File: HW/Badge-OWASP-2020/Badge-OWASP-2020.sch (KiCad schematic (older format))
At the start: 18 parts

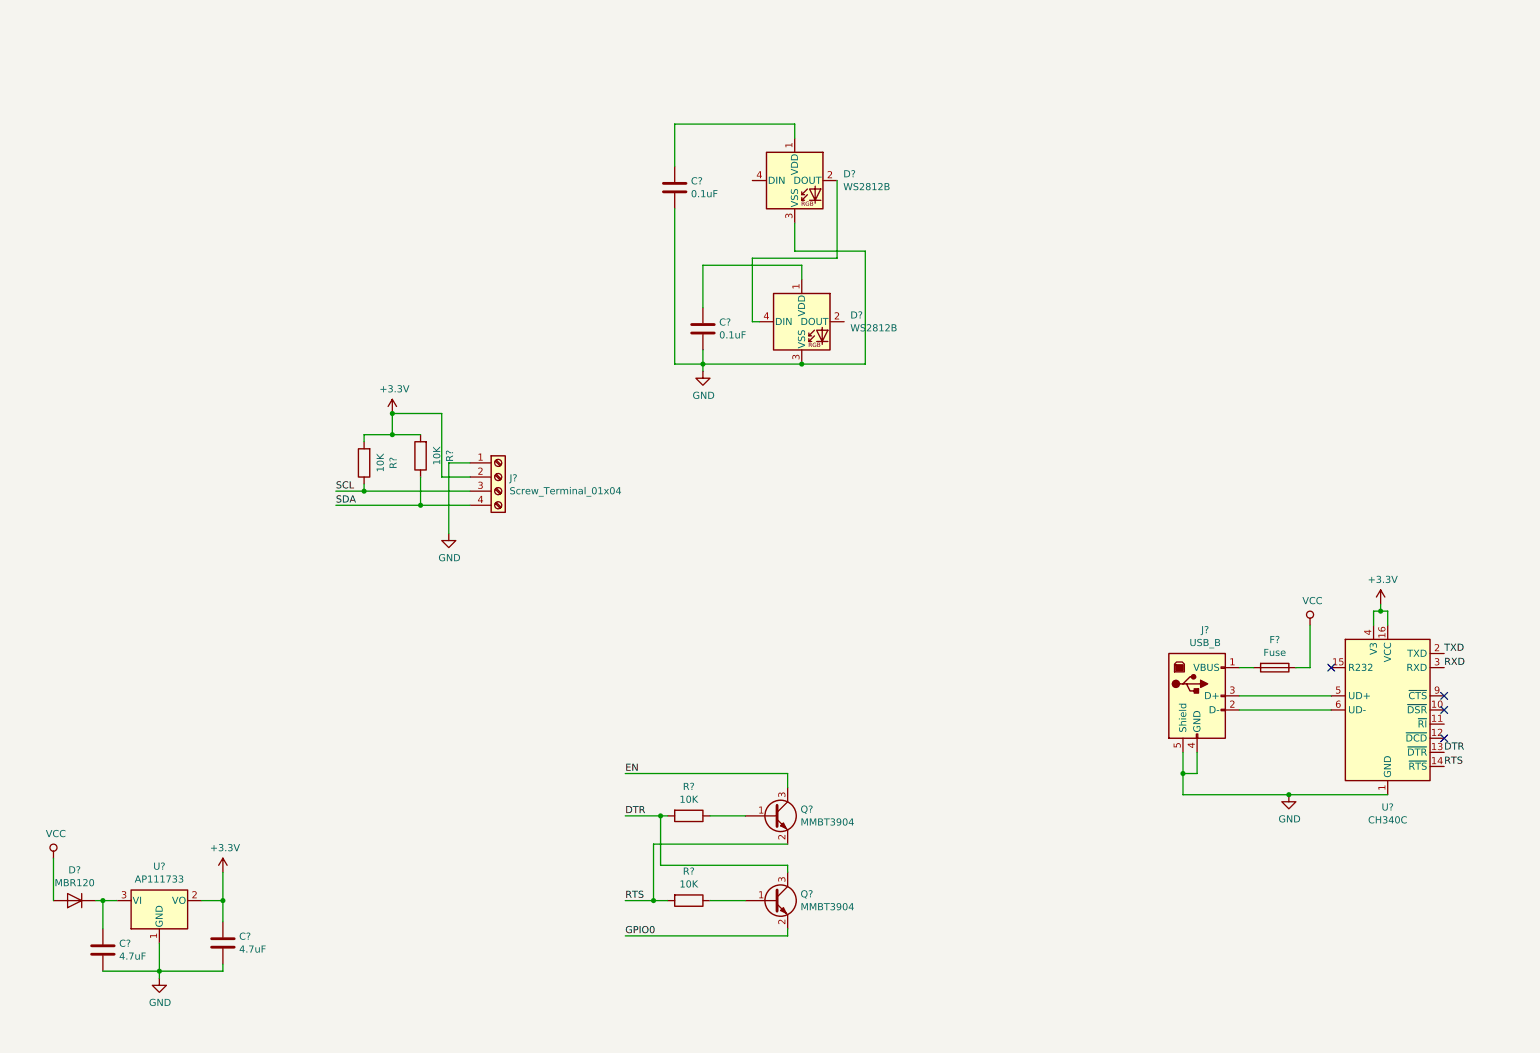
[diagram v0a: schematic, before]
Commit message: ESP32
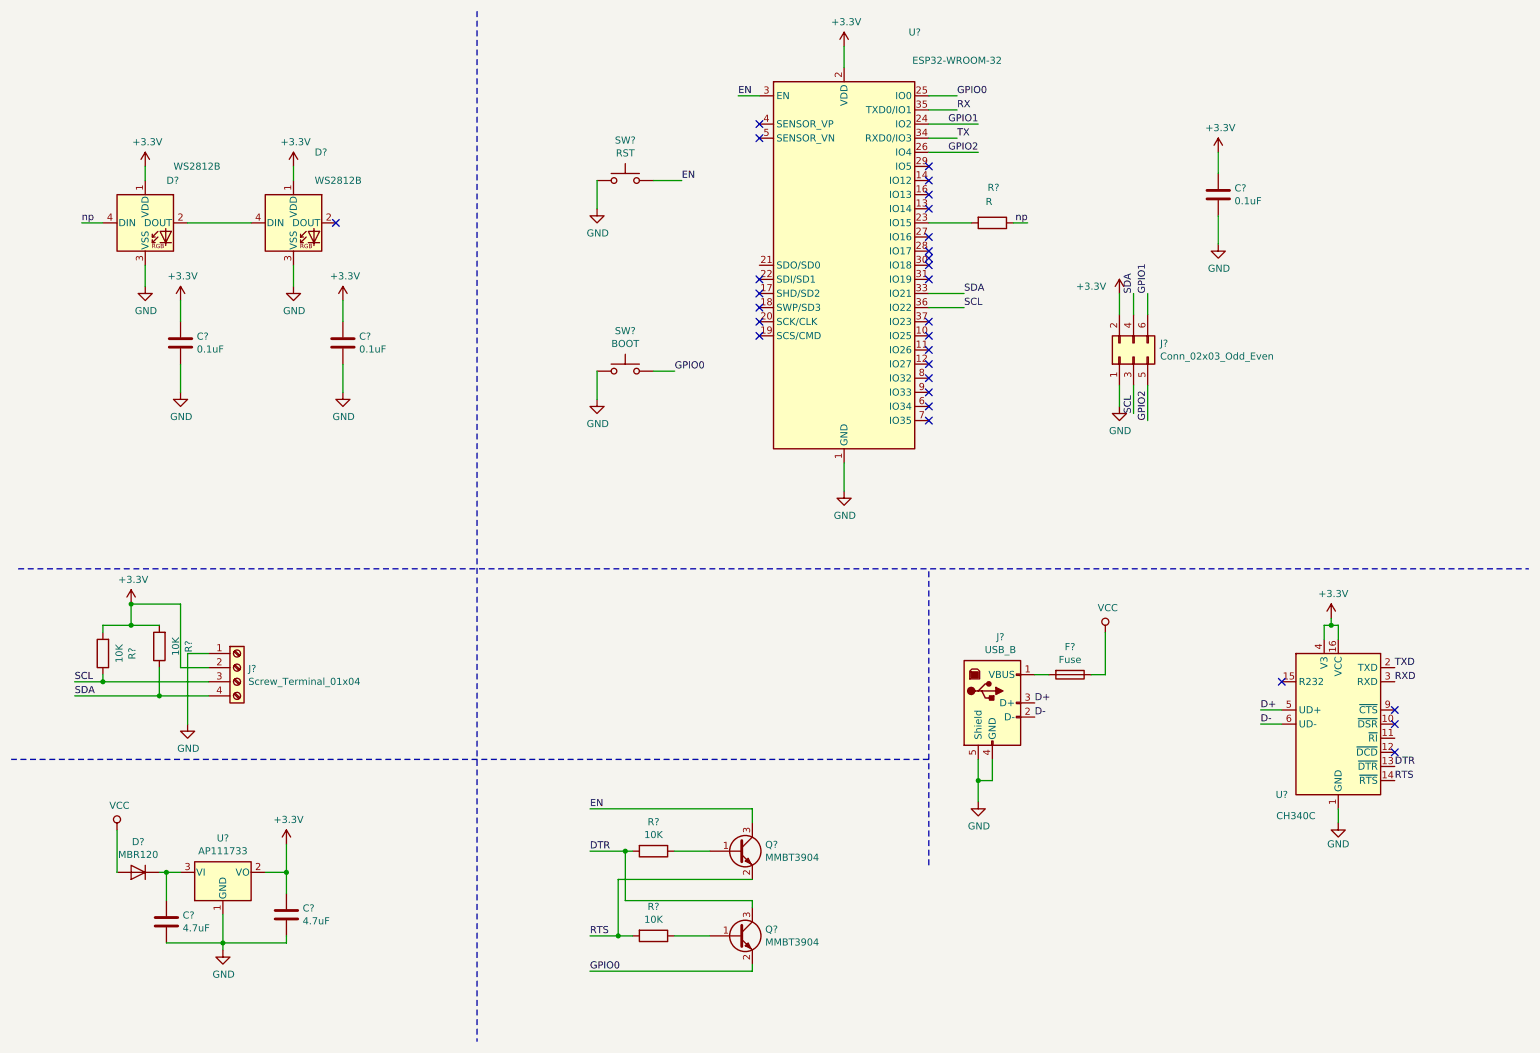
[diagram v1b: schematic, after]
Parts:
- added C?: 0.1uF, symbol Device:C
- added J?: Conn_02x03_Odd_Even, symbol Connector_Generic:Conn_02x03_Odd_Even
- added R?: R, symbol Device:R
- added SW?: RST, symbol Switch:SW_Push
- added SW?: BOOT, symbol Switch:SW_Push
- added U?: ESP32-WROOM-32, RF_Module:ESP32-WROOM-32, symbol RF_Module:ESP32-WROOM-32
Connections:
- net +3V3: now also C?.1, C?.1, D?.1 (VDD), D?.1 (VDD), C?.1, J?.2 (Pin_2), U?.2 (VDD)
- net EN: now also SW?.2, U?.3 (EN)
- net GND: now also C?.2, J?.1 (Pin_1), SW?.1, SW?.1, U?.1 (GND), U?.15 (GND), U?.38 (GND)
- net GPIO0: now also SW?.2, U?.25 (IO0)
- net SCL: now also J?.3 (Pin_3), U?.36 (IO22)
- net SDA: now also J?.4 (Pin_4), U?.33 (IO21)
- net D+: now reaches J?.3 (D+), U?.5 (UD+)
- net D-: now reaches J?.2 (D-), U?.6 (UD-)
- net np: now reaches D?.4 (DIN)
- net np: now also R?.1
- new net: R?.2, U?.23 (IO15)
- new net GPIO1: J?.6 (Pin_6), U?.24 (IO2)
- new net GPIO2: J?.5 (Pin_5), U?.26 (IO4)
- new net RX: U?.35 (TXD0/IO1)
- new net TX: U?.34 (RXD0/IO3)
- no-connect marks 4 -> 29
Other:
- moved on the sheet: C?, D?, F?, J?, Q?, R?, U?
